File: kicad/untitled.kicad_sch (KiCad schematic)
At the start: 10 parts, among them J3 AVR-ISP-6, J4 AVR-ISP-6, J5 AVR-ISP-6, M1 Motor_DC, Q1 NMOS, U3 ATmega328P-P, U4 ATmega328P-P, U5 ATmega328P-P

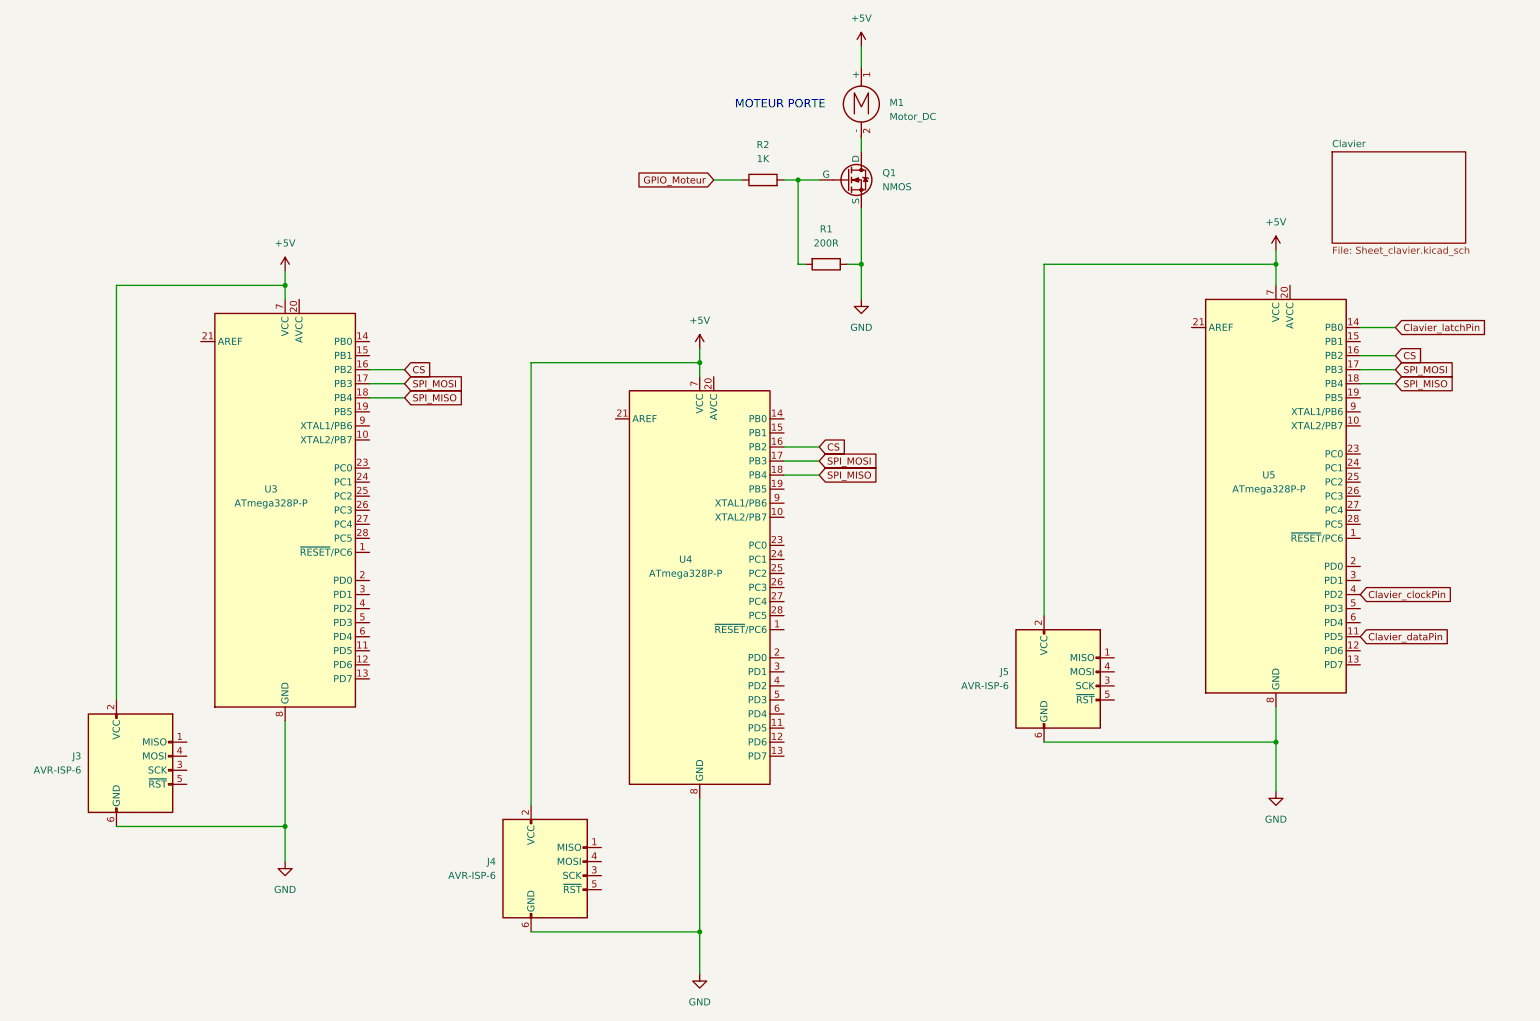
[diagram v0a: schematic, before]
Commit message: update sur tout le schema
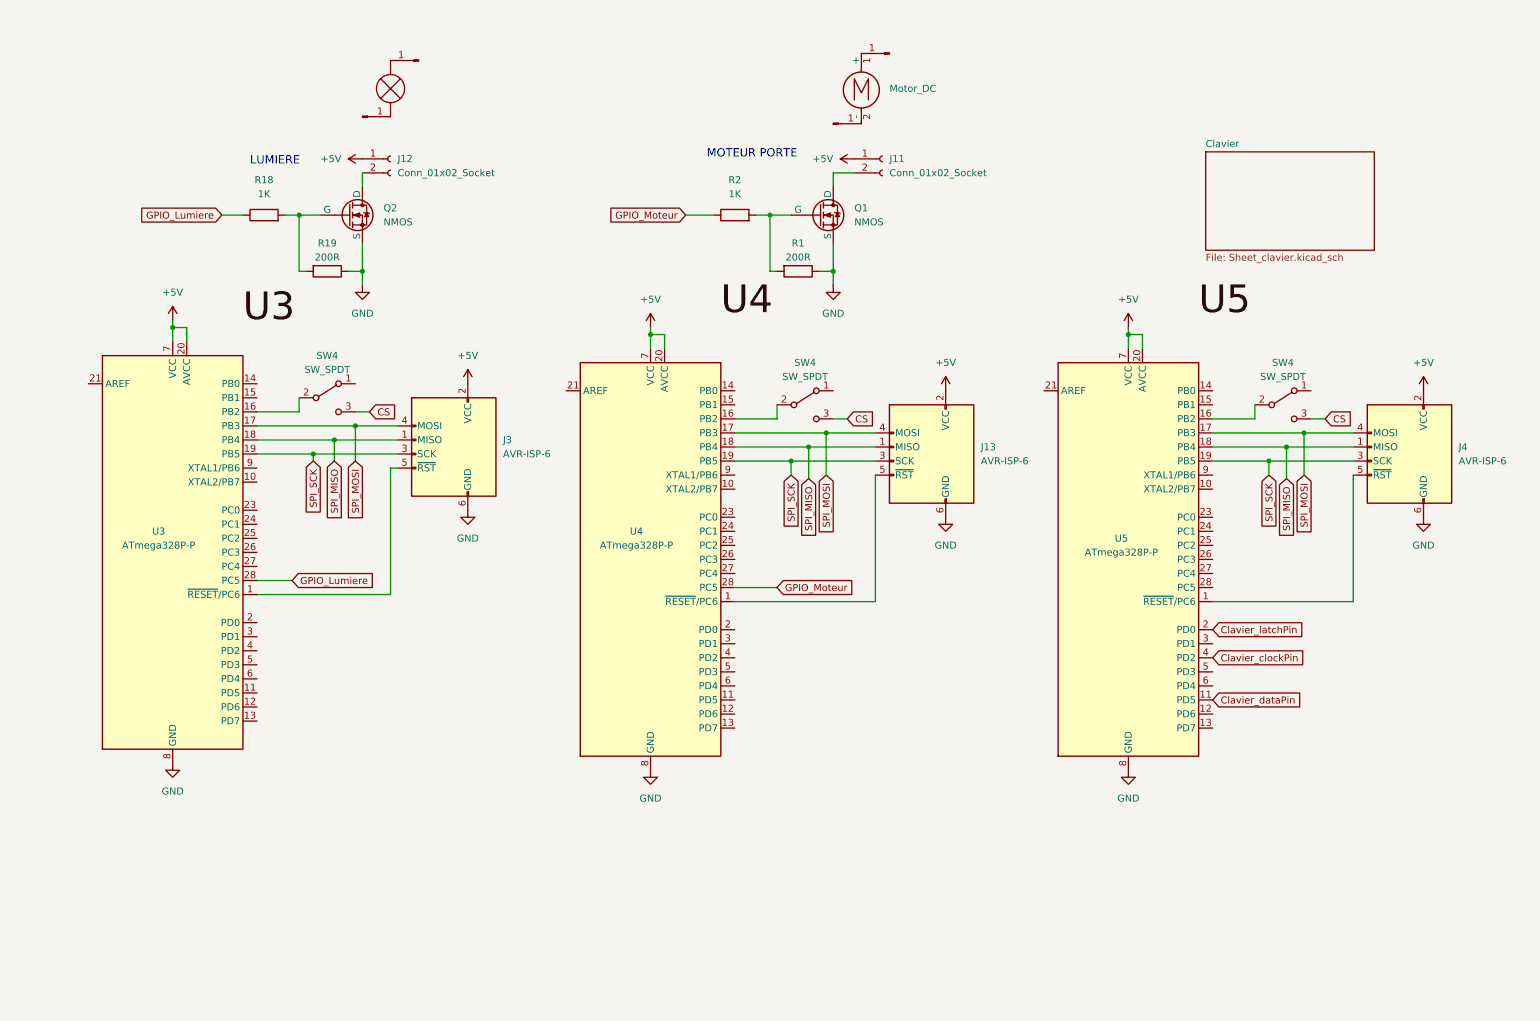
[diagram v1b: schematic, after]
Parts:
- removed J5: AVR-ISP-6, Connector_IDC:IDC-Header_2x03_P2.54mm_Vertical, symbol Connector:AVR-ISP-6
- added J11, J12: Conn_01x02_Socket, symbol Connector:Conn_01x02_Socket
- added J13: AVR-ISP-6, Connector_IDC:IDC-Header_2x03_P2.54mm_Vertical, symbol Connector:AVR-ISP-6
- added J6, J7, J8, J9: Conn_01x01_Pin, symbol Connector:Conn_01x01_Pin
- added LA1: Lamp, symbol Device:Lamp
- added Q2: NMOS, symbol Simulation_SPICE:NMOS
- added R18: 1K, symbol Device:R
- added R19: 200R, symbol Device:R
- added SW4 (x3): SW_SPDT, symbol Switch:SW_SPDT
- M1: now left out of the parts list
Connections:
- net +5V: now also U3.20 (AVCC), U4.20 (AVCC), U5.20 (AVCC), J11.1 (Pin_1), J12.1 (Pin_1), J13.2 (VCC); no longer M1.1 (+)
- net CS: now also SW4.3 (C), SW4.3 (C), SW4.3 (C); no longer U3.16 (PB2), U4.16 (PB2), U5.16 (PB2)
- net Clavier_latchPin: now also U5.2 (PD0); no longer U5.14 (PB0)
- net GND: now also J13.6 (GND), Q2.3 (S), R19.1
- net GPIO_Moteur: now also U4.28 (PC5)
- net SPI_MISO: now also J3.1 (MISO), J4.1 (MISO), J13.1 (MISO)
- net SPI_MOSI: now also J3.4 (MOSI), J4.4 (MOSI), J13.4 (MOSI)
- net at U3.1 (~{RESET}/PC6): now also J3.5 (~{RST})
- net SPI_SCK: now reaches U3.19 (PB5)
- net SPI_SCK: now also J3.3 (SCK), J4.3 (SCK), U4.19 (PB5), U5.19 (PB5), J13.3 (SCK)
- net GPIO_Lumiere: now reaches U3.28 (PC5)
- net GPIO_Lumiere: now also R18.1
- net at U4.1 (~{RESET}/PC6): now also J13.5 (~{RST})
- net at Q1.1 (D): now also J11.2 (Pin_2); no longer M1.2 (-)
- net at U5.1 (~{RESET}/PC6): now also J4.5 (~{RST})
- new net: J7.1 (Pin_1), LA1.1 (-)
- new net: J6.1 (Pin_1), LA1.2 (+)
- new net: SW4.2 (B), U4.16 (PB2)
- new net: SW4.2 (B), U3.16 (PB2)
- new net: J12.2 (Pin_2), Q2.1 (D)
- new net: Q2.2 (G), R18.2, R19.2
- new net: J9.1 (Pin_1), M1.2 (-)
- new net: SW4.2 (B), U5.16 (PB2)
- new net: J8.1 (Pin_1), M1.1 (+)
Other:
- note added: "LUMIERE"
- moved on the sheet: Q1, R1, R2, U3, U4, U5

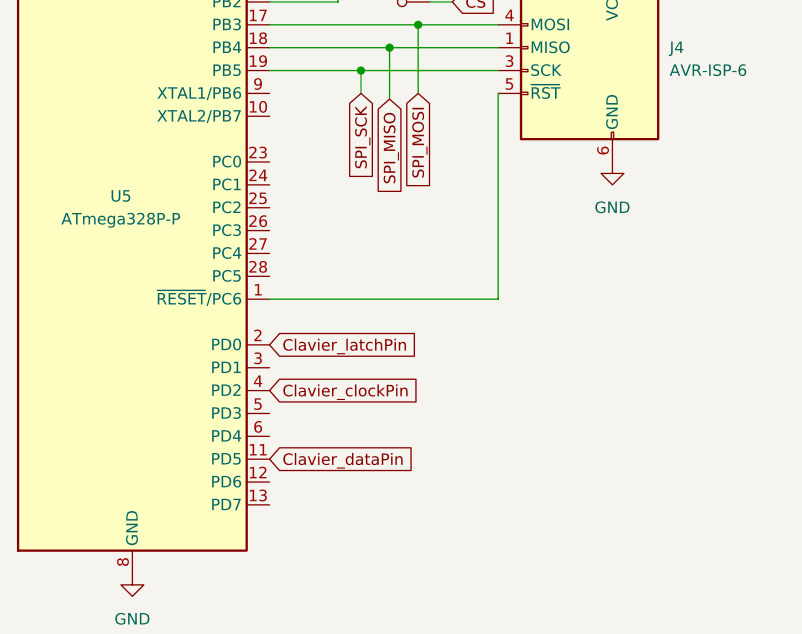
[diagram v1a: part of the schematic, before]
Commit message: updates clavier
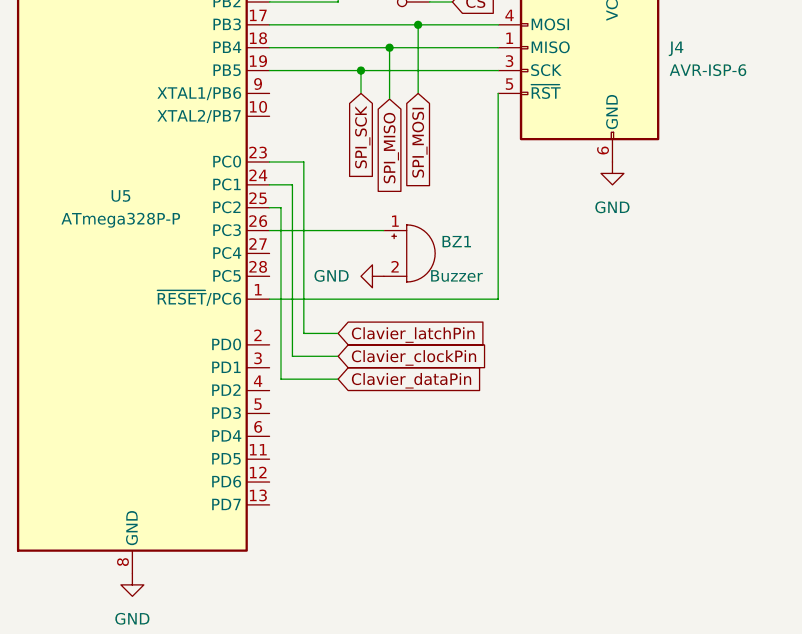
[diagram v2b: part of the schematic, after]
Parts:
- added BZ1: Buzzer, symbol Device:Buzzer
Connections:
- net Clavier_clockPin: now also U5.24 (PC1); no longer U5.4 (PD2)
- net Clavier_dataPin: now also U5.25 (PC2); no longer U5.11 (PD5)
- net Clavier_latchPin: now also U5.23 (PC0); no longer U5.2 (PD0)
- net GND: now also BZ1.2 (+)
- net at U5.26 (PC3): now also BZ1.1 (-)
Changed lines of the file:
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@@
+    (stroke (width 0) (type default))
+  )
+  (wire (pts (xy 232.41 127) (xy 232.41 107.95))
     (stroke (width 0) (type default))
   )
@@
     (stroke (width 0) (type default))
   )
+  (wire (pts (xy 231.14 129.54) (xy 231.14 110.49))
+    (stroke (width 0) (type default))
+  )
   (wire (pts (xy 167.64 100.33) (xy 167.64 123.19))
     (stroke (width 0) (type default))
   )
+  (wire (pts (xy 228.6 115.57) (xy 241.3 115.57))
+    (stroke (width 0) (type default))
+  )
   (wire (pts (xy 43.18 73.66) (xy 40.64 73.66))
     (stroke (width 0) (type default))
@@
     (stroke (width 0) (type default))
   )
+  (wire (pts (xy 229.87 132.08) (xy 229.87 113.03))
+    (stroke (width 0) (type default))
+  )
   (wire (pts (xy 63.5 53.34) (xy 67.31 53.34))
     (stroke (width 0) (type default))
@@
     (stroke (width 0) (type default))
   )
+  (wire (pts (xy 236.22 127) (xy 232.41 127))
+    (stroke (width 0) (type default))
+  )
   (wire (pts (xy 228.6 90.17) (xy 236.22 90.17))
     (stroke (width 0) (type default))
@@
     (stroke (width 0) (type default))
   )
+  (wire (pts (xy 236.22 132.08) (xy 229.87 132.08))
+    (stroke (width 0) (type default))
+  )
   (wire (pts (xy 158.75 92.71) (xy 167.64 92.71))
     (stroke (width 0) (type default))
@@
     (stroke (width 0) (type default))
   )
+  (wire (pts (xy 229.87 113.03) (xy 228.6 113.03))
+    (stroke (width 0) (type default))
+  )
   (wire (pts (xy 160.02 63.5) (xy 160.02 66.04))
     (stroke (width 0) (type default))
@@
     (stroke (width 0) (type default))
   )
+  (wire (pts (xy 232.41 107.95) (xy 228.6 107.95))
+    (stroke (width 0) (type default))
+  )
   (wire (pts (xy 73.66 91.44) (xy 81.28 91.44))
     (stroke (width 0) (type default))
   )
+  (wire (pts (xy 236.22 129.54) (xy 231.14 129.54))
+    (stroke (width 0) (type default))
+  )
   (wire (pts (xy 160.02 58.42) (xy 160.02 63.5))
     (stroke (width 0) (type default))
@@
   )
   (wire (pts (xy 245.11 100.33) (xy 245.11 92.71))
+    (stroke (width 0) (type default))
+  )
+  (wire (pts (xy 231.14 110.49) (xy 228.6 110.49))
     (stroke (width 0) (type default))
   )
@@
     )
   )
-  (global_label "Clavier_clockPin" (shape input) (at 228.6 133.35 0) (fields_autoplaced)
+  (global_label "Clavier_clockPin" (shape input) (at 236.22 129.54 0) (fields_autoplaced)
     (effects (font (size 1.27 1.27)) (justify left))
-    (property "Intersheetrefs" "${INTERSHEET_REFS}" (at 247.0481 133.35 0)
+    (property "Intersheetrefs" "${INTERSHEET_REFS}" (at 254.6681 129.54 0)
       (effects (font (size 1.27 1.27)) (justify left) hide)
     )
@@
     )
   )
-  (global_label "Clavier_latchPin" (shape input) (at 228.6 128.27 0) (fields_autoplaced)
+  (global_label "Clavier_latchPin" (shape input) (at 236.22 127 0) (fields_autoplaced)
     (effects (font (size 1.27 1.27)) (justify left))
-    (property "Intersheetrefs" "${INTERSHEET_REFS}" (at 246.8061 128.27 0)
+    (property "Intersheetrefs" "${INTERSHEET_REFS}" (at 254.4261 127 0)
       (effects (font (size 1.27 1.27)) (justify left) hide)
     )
@@
     )
   )
-  (global_label "Clavier_dataPin" (shape input) (at 228.6 140.97 0) (fields_autoplaced)
+  (global_label "Clavier_dataPin" (shape input) (at 236.22 132.08 0) (fields_autoplaced)
     (effects (font (size 1.27 1.27)) (justify left))
-    (property "Intersheetrefs" "${INTERSHEET_REFS}" (at 246.2013 140.97 0)
+    (property "Intersheetrefs" "${INTERSHEET_REFS}" (at 253.8213 132.08 0)
       (effects (font (size 1.27 1.27)) (justify left) hide)
     )
@@
     )
   )
+  (symbol (lib_id "power:GND") (at 241.3 120.65 270) (unit 1)
+    (in_bom yes) (on_board yes) (dnp no) (fields_autoplaced)
+    (property "Reference" "#PWR049" (at 234.95 120.65 0)
+      (effects (font (size 1.27 1.27)) hide)
+    )
+    (property "Value" "GND" (at 237.49 120.65 90)
+      (effects (font (size 1.27 1.27)) (justify right))
+    )
+    (property "Footprint" "" (at 241.3 120.65 0)
+      (effects (font (size 1.27 1.27)) hide)
+    )
+    (property "Datasheet" "" (at 241.3 120.65 0)
+      (effects (font (size 1.27 1.27)) hide)
+    )
+    (pin "1")
+    (instances
+      (project "MaisonEtape1"
+        (path "/ed06f8de-d1bb-4b1a-bfe3-5df11d3a9162"
+          (reference "#PWR049") (unit 1)
+        )
+        (path "/ed06f8de-d1bb-4b1a-bfe3-5df11d3a9162/0600536b-f413-4b06-98e9-b5748b5de992"
+          (reference "#PWR055") (unit 1)
+        )
+      )
+    )
+  )
   (symbol (lib_id "MCU_Microchip_ATmega:ATmega328P-P") (at 127 115.57 0) (unit 1)
     (in_bom yes) (on_board yes) (dnp no)
@@
         )
       )
+    )
+  )
+  (symbol (lib_id "Device:Buzzer") (at 243.84 118.11 0) (unit 1)
+    (in_bom yes) (on_board yes) (dnp no)
+    (property "Reference" "BZ1" (at 247.65 116.84 0)
+      (effects (font (size 1.27 1.27)) (justify left))
+    )
+    (property "Value" "Buzzer" (at 246.38 120.65 0)
+      (effects (font (size 1.27 1.27)) (justify left))
+    )
+    (property "Footprint" "" (at 243.205 115.57 90)
+      (effects (font (size 1.27 1.27)) hide)
+    )
+    (property "Datasheet" "~" (at 243.205 115.57 90)
+      (effects (font (size 1.27 1.27)) hide)
+    )
+    (pin "1")
+    (pin "2")
+    (instances
+      (project "MaisonEtape1"
+        (path "/ed06f8de-d1bb-4b1a-bfe3-5df11d3a9162/0600536b-f413-4b06-98e9-b5748b5de992"
+          (reference "BZ1") (unit 1)
+        )
+      )
